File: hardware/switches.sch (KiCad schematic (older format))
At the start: 11 parts, among them P5 USB_A_2, Q2 Q_NMOS_GSD, Q3 Q_PMOS_GSD, U10 touchpad, U4 housing-mounts

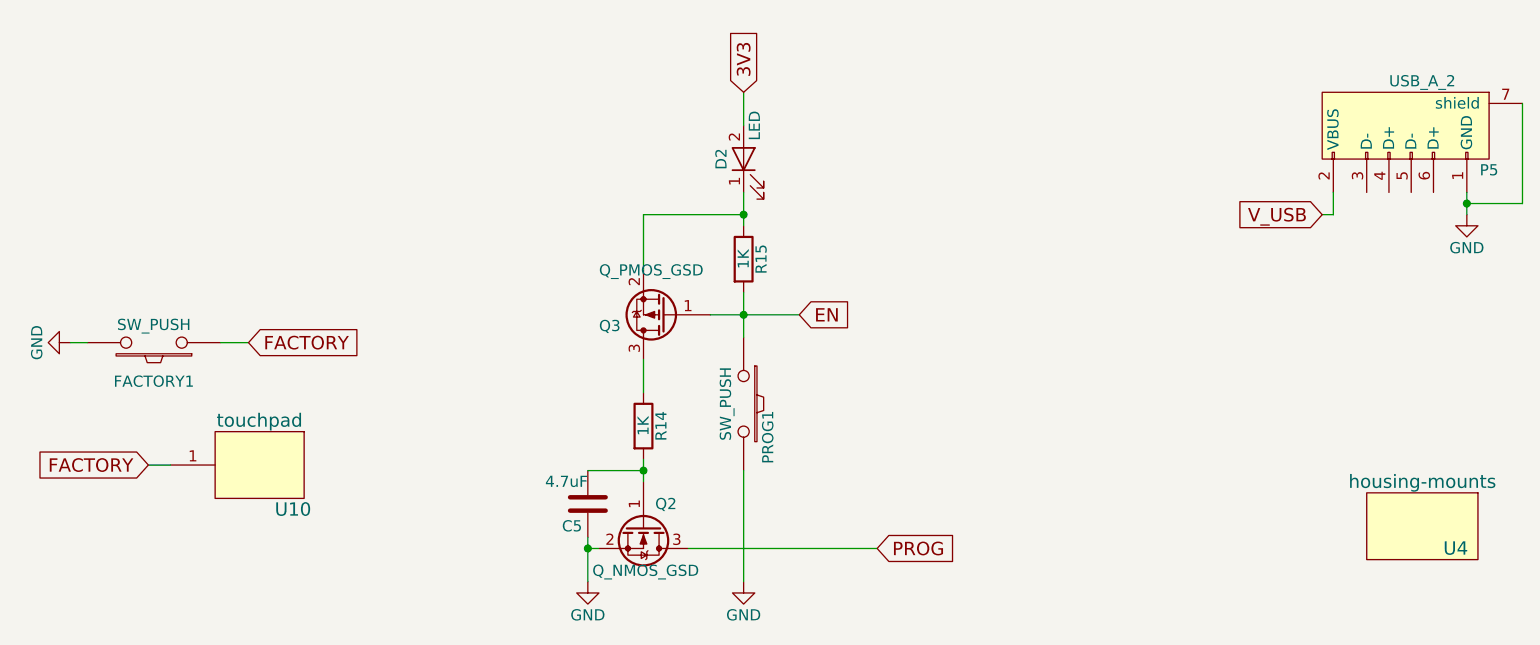
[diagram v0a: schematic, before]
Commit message: update
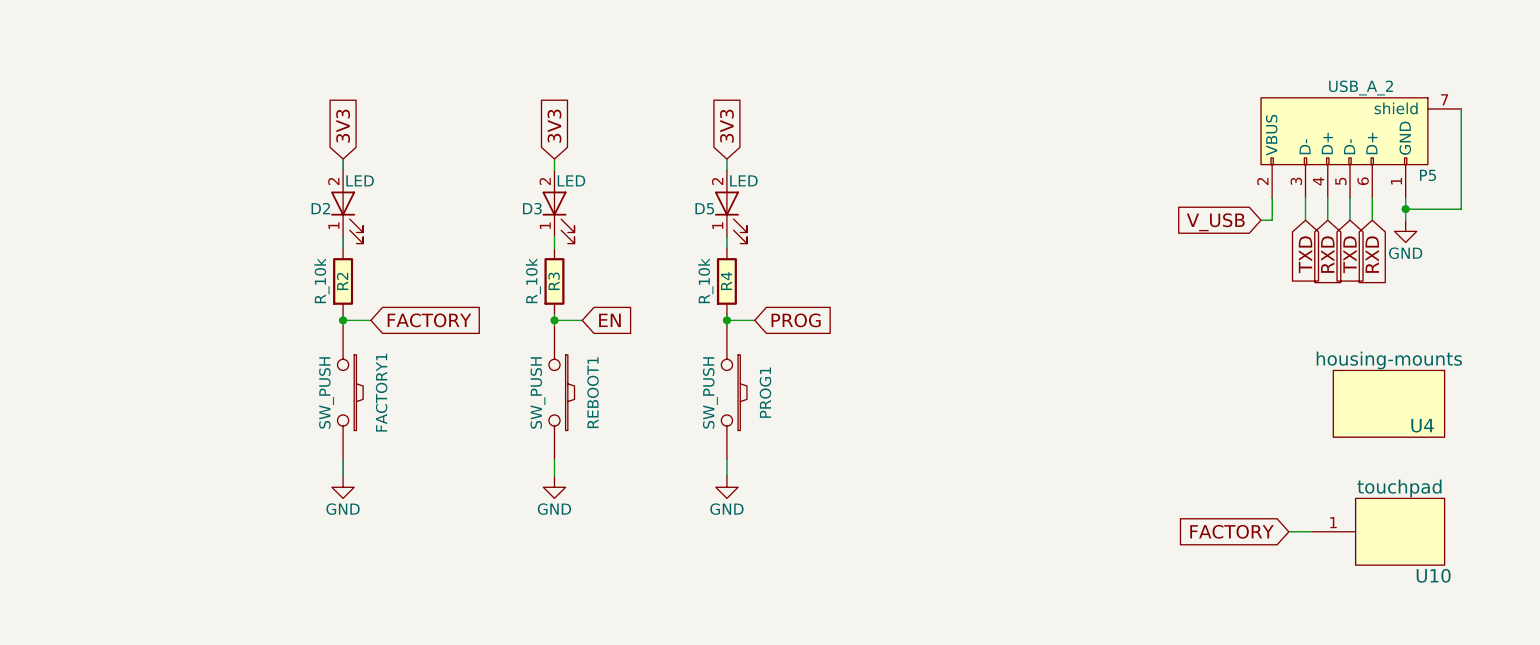
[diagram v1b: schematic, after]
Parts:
- removed C5: 4.7uF, Capacitors_SMD:C_0603_HandSoldering, symbol C
- removed Q2: Q_NMOS_GSD, TO_SOT_Packages_SMD:SOT-23, symbol Q_NMOS_GSD
- removed Q3: Q_PMOS_GSD, TO_SOT_Packages_SMD:SOT-23, symbol Q_PMOS_GSD
- removed R14, R15: 1K, Resistors_SMD:R_0603_HandSoldering, symbol R
- added D3, D5: LED, LEDs:LED_0603, symbol LED
- added R2, R3, R4: R_10k, Resistors_SMD:R_0603_HandSoldering, symbol R_10k
- added REBOOT1: SW_PUSH, Buttons_Switches_SMD:SW_SPST_KMR2, symbol SW_PUSH
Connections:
- net 3V3: now also D3.2 (A), D5.2 (A)
- net EN: now also R3.2, REBOOT1.1; no longer PROG1.1
- net FACTORY: now also R2.2
- net GND: now also REBOOT1.2
- net PROG: now also PROG1.1, R4.2
- net at D2.1 (K): now also R2.1
- net TXD: now reaches P5.3 (D-)
- net TXD: now also P5.5 (D-)
- net RXD: now reaches P5.4 (D+)
- net RXD: now also P5.6 (D+)
- new net: D3.1 (K), R3.1
- new net: D5.1 (K), R4.1
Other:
- moved on the sheet: D2, FACTORY1, P5, U10, U4

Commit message: update
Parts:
- D2, D3, D5: footprint LEDs:LED_0603 -> LEDs:LED_0603_HandSoldering
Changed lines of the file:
@@
 F 0 "D2" V 3700 3225 50  0000 C CNN
 F 1 "LED" V 3825 3050 50  0000 C CNN
-F 2 "LEDs:LED_0603" H 3725 3125 50  0001 C CNN
+F 2 "LEDs:LED_0603_HandSoldering" H 3725 3125 50  0001 C CNN
 F 3 "http://www.osram-os.com/Graphics/XPic9/00128792_0.pdf" H 3725 3125 50  0001 C CNN
 F 4 "475-2512-2-ND" H 3725 3125 60  0001 C CNN "Part Number"
@@
 F 0 "D3" V 4650 3225 50  0000 C CNN
 F 1 "LED" V 4775 3050 50  0000 C CNN
-F 2 "LEDs:LED_0603" H 4675 3125 50  0001 C CNN
+F 2 "LEDs:LED_0603_HandSoldering" H 4675 3125 50  0001 C CNN
 F 3 "http://www.osram-os.com/Graphics/XPic9/00128792_0.pdf" H 4675 3125 50  0001 C CNN
 F 4 "475-2512-2-ND" H 4675 3125 60  0001 C CNN "Part Number"
@@
 F 0 "D5" V 5425 3225 50  0000 C CNN
 F 1 "LED" V 5550 3050 50  0000 C CNN
-F 2 "LEDs:LED_0603" H 5450 3125 50  0001 C CNN
+F 2 "LEDs:LED_0603_HandSoldering" H 5450 3125 50  0001 C CNN
 F 3 "http://www.osram-os.com/Graphics/XPic9/00128792_0.pdf" H 5450 3125 50  0001 C CNN
 F 4 "475-2512-2-ND" H 5450 3125 60  0001 C CNN "Part Number"
